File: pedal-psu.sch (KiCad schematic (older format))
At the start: 65 parts, among them J1 Conn_01x01_Male, J2 Conn_01x01_Male, J3 Conn_01x02_Male, J4 Conn_01x02_Male, J5 Conn_01x02_Male, J6 Conn_01x02_Male, T1 Transformer_1P_1S, T2 Transformer_1P_1S, U1 LM7809_TO220, U2 LM324, U4 LM7805_TO220, U5 LM317_3PinPackage

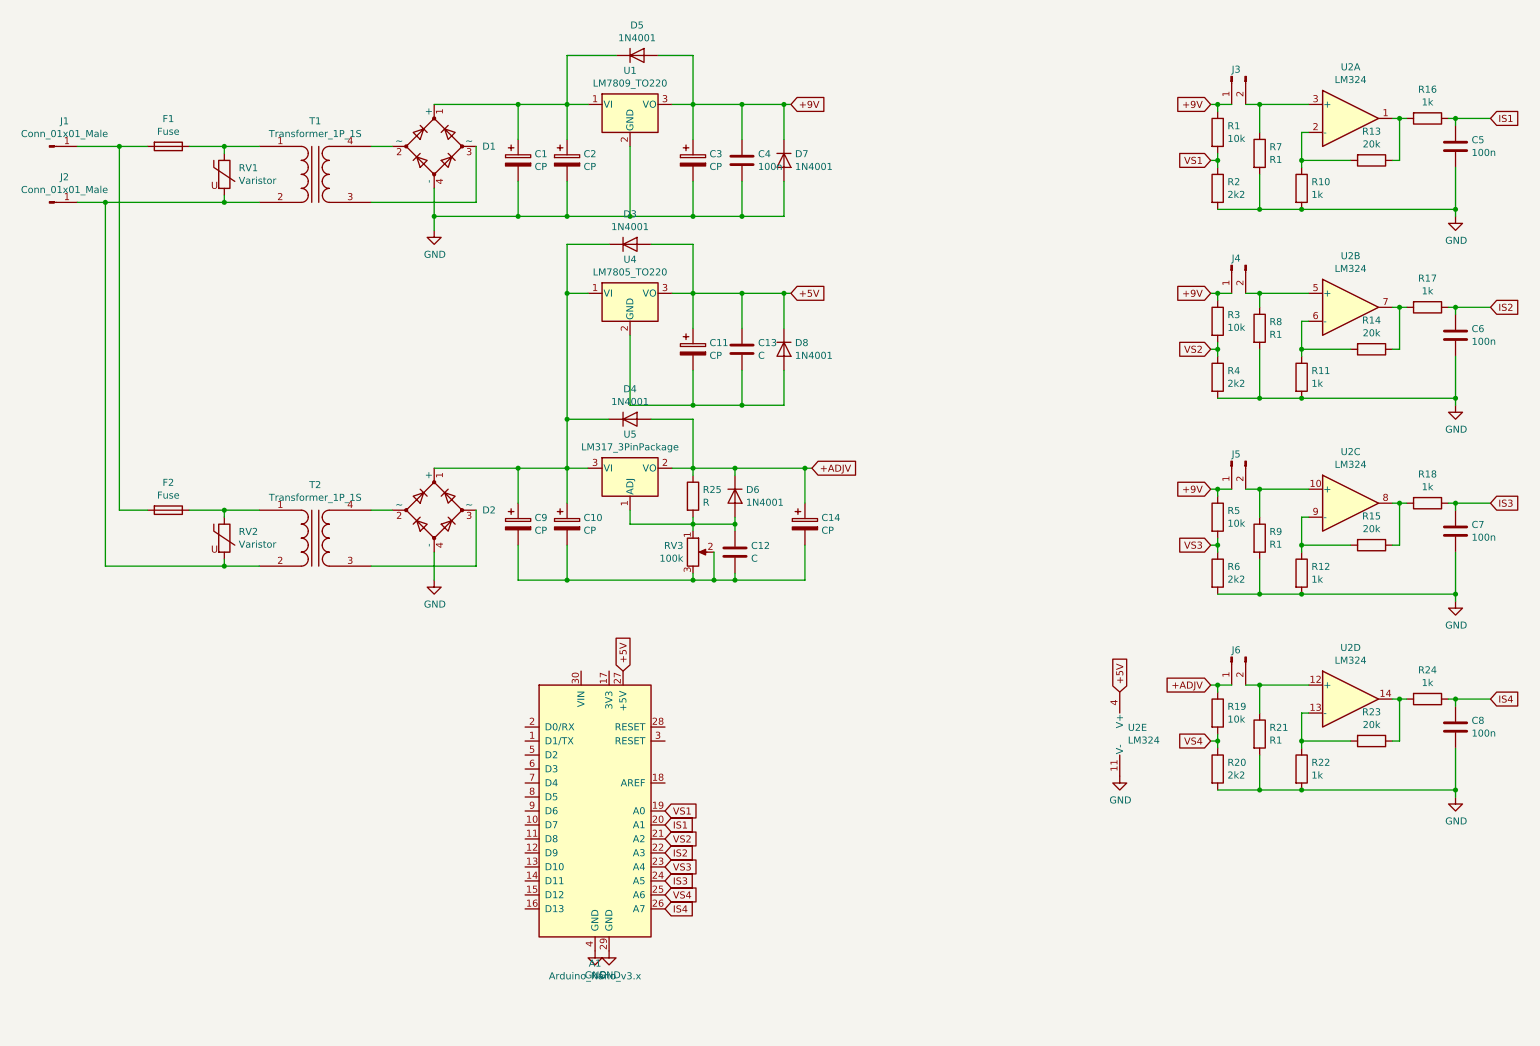
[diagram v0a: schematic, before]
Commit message: Complete schematic, moving on to PCB design.
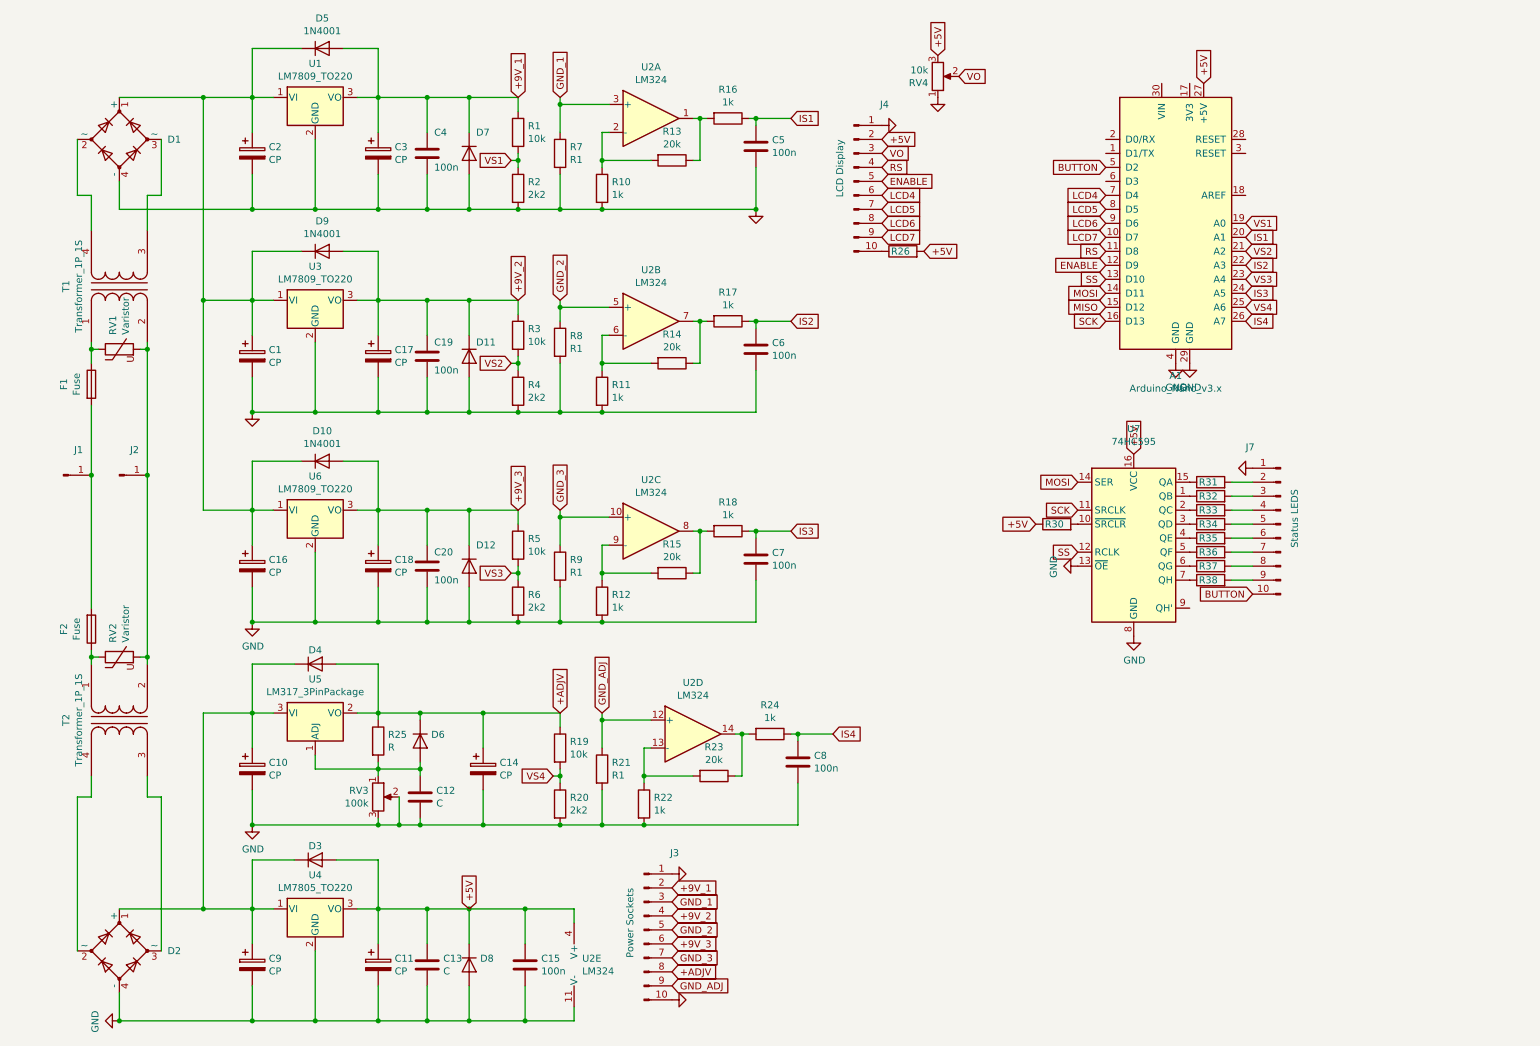
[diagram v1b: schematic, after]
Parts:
- removed J3, J4, J5, J6: Conn_01x02_Male, Connector_Molex:Molex_KK-254_AE-6410-02A_1x02_P2.54mm_Vertical, symbol Connector:Conn_01x02_Male
- added C15, C19, C20: 100n, Capacitor_SMD:C_1210_3225Metric_Pad1.42x2.65mm_HandSolder, symbol Device:C
- added C16: CP, Capacitor_THT:C_Radial_D10.0mm_H12.5mm_P5.00mm, symbol Device:CP
- added C17, C18: CP, Capacitor_THT:C_Radial_D6.3mm_H5.0mm_P2.50mm, symbol Device:CP
- added D10, D11, D12, D9: 1N4001, Diode_SMD:D_SMA_Handsoldering, symbol Diode:1N4001
- added J3: Power Sockets, Connector_Molex:Molex_KK-254_AE-6410-10A_1x10_P2.54mm_Vertical, symbol Connector:Conn_01x10_Male
- added J4: LCD Display, Connector_Molex:Molex_KK-254_AE-6410-10A_1x10_P2.54mm_Vertical, symbol Connector:Conn_01x10_Male
- added J7: Status LEDS, Connector_Molex:Molex_KK-254_AE-6410-10A_1x10_P2.54mm_Vertical, symbol Connector:Conn_01x10_Male
- added R26: 220, Resistor_SMD:R_0805_2012Metric_Pad1.15x1.40mm_HandSolder, symbol Device:R
- added R30: 100k, Resistor_SMD:R_0805_2012Metric_Pad1.15x1.40mm_HandSolder, symbol Device:R
- added R31, R32, R33, R34, R35, R36, R37, R38: 560, Resistor_SMD:R_0805_2012Metric_Pad1.15x1.40mm_HandSolder, symbol Device:R
- added RV4: 10k, Potentiometer_THT:Potentiometer_Piher_PT-6-V_Vertical, symbol Device:R_POT
- added U3, U6: LM7809_TO220, Package_TO_SOT_THT:TO-220-3_Vertical, symbol Regulator_Linear:LM7809_TO220
- added U7: 74HC595, Package_SO:SOP-16_4.4x10.4mm_P1.27mm, symbol 74xx:74HC595
- T1, T2: footprint Transformer_THT:Transformer_CHK_EI42-5VA_1xSec -> pedal-psu:Transformer_V42AJ
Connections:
- net +5V: now also C15.1, J4.2 (Pin_2), R26.2, R30.1, RV4.3, U7.16 (VCC)
- net +ADJV: now also J3.8 (Pin_8)
- net GND: now also C10.2, C11.2, C12.2, C13.2, C14.2, C9.2, D8.2 (A), RV3.2, RV3.3, U4.2 (GND), C15.2, C16.2, C17.2, C18.2, C19.2, C20.2, D11.2 (A), D12.2 (A), J3.1 (Pin_1), J3.10 (Pin_10), J4.1 (Pin_1), J7.1 (Pin_1), RV4.1, U3.2 (GND), U6.2 (GND), U7.13 (~OE), U7.8 (GND)
- net at C1.1, C2.1, D1.1 (+)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: now also C16.1, D10.1 (K), D9.1 (K), U3.1 (VI), U6.1 (VI)
- net GND_2: now reaches R8.1, U2.5 (+)
- net GND_2: now also J3.5 (Pin_5)
- net GND_1: now reaches R7.1, U2.3 (+)
- net GND_1: now also J3.3 (Pin_3)
- net GND_3: now reaches R9.1, U2.10 (+)
- net GND_3: now also J3.7 (Pin_7)
- net GND_ADJ: now reaches R21.1, U2.12 (+)
- net GND_ADJ: now also J3.9 (Pin_9)
- net LCD7: now reaches A1.10 (D7)
- net LCD7: now also J4.9 (Pin_9)
- net RS: now reaches A1.11 (D8)
- net RS: now also J4.4 (Pin_4)
- net ENABLE: now reaches A1.12 (D9)
- net ENABLE: now also J4.5 (Pin_5)
- net SS: now reaches A1.13 (D10)
- net SS: now also U7.12 (RCLK)
- net MOSI: now reaches A1.14 (D11)
- net MOSI: now also U7.14 (SER)
- net MISO: now reaches A1.15 (D12)
- net SCK: now reaches A1.16 (D13)
- net SCK: now also U7.11 (SRCLK)
- net BUTTON: now reaches A1.5 (D2)
- net BUTTON: now also J7.10 (Pin_10)
- net LCD4: now reaches A1.7 (D4)
- net LCD4: now also J4.6 (Pin_6)
- net LCD5: now reaches A1.8 (D5)
- net LCD5: now also J4.7 (Pin_7)
- net LCD6: now reaches A1.9 (D6)
- net LCD6: now also J4.8 (Pin_8)
- net +9V renamed +9V_1
- net +9V_1: now also J3.2 (Pin_2); no longer R3.1, R5.1
- new net: R32.1, U7.1 (QB)
- new net: R30.2, U7.10 (~SRCLR)
- new net: R31.1, U7.15 (QA)
- new net: R33.1, U7.2 (QC)
- new net: R34.1, U7.3 (QD)
- new net: R35.1, U7.4 (QE)
- new net: R36.1, U7.5 (QF)
- new net: R37.1, U7.6 (QG)
- new net: R38.1, U7.7 (QH)
- new net: J7.2 (Pin_2), R31.2
- new net: J7.3 (Pin_3), R32.2
- new net: J7.4 (Pin_4), R33.2
- new net: J7.5 (Pin_5), R34.2
- new net: J7.6 (Pin_6), R35.2
- new net: J7.7 (Pin_7), R36.2
- new net: J7.8 (Pin_8), R37.2
- new net: J7.9 (Pin_9), R38.2
- new net: J4.10 (Pin_10), R26.1
- new net +9V_2: C17.1, C19.1, D11.1 (K), D9.2 (A), J3.4 (Pin_4), R3.1, U3.3 (VO)
- new net +9V_3: C18.1, C20.1, D10.2 (A), D12.1 (K), J3.6 (Pin_6), R5.1, U6.3 (VO)
- new net VO: J4.3 (Pin_3), RV4.2
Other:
- moved on the sheet: A1, C1, C10, C11, C12, C13, C14, C2, C3, C4, C5, C6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
